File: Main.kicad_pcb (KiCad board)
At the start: 2 copper layers, 71.3 x 94.1 mm, 50 parts, among them J1 Conn_01x02, J10 Conn_01x04, J11 Conn_01x02, J12 Conn_01x02, J13 Conn_01x02, J14 Conn_01x02, J15 Conn_01x02, J2 Conn_01x02, J3 Conn_01x04, J4 Conn_01x02, J5 Conn_01x02, J6 Conn_01x08_Socket, J7 Conn_01x08_Socket, J8 Conn_01x08_Socket, J9 Conn_01x08_Socket, Q1 PMOS, Q2 SS8050, U1 DEV-16771, U2 K230D, U4 AP63201WU, U6 AP63201WU

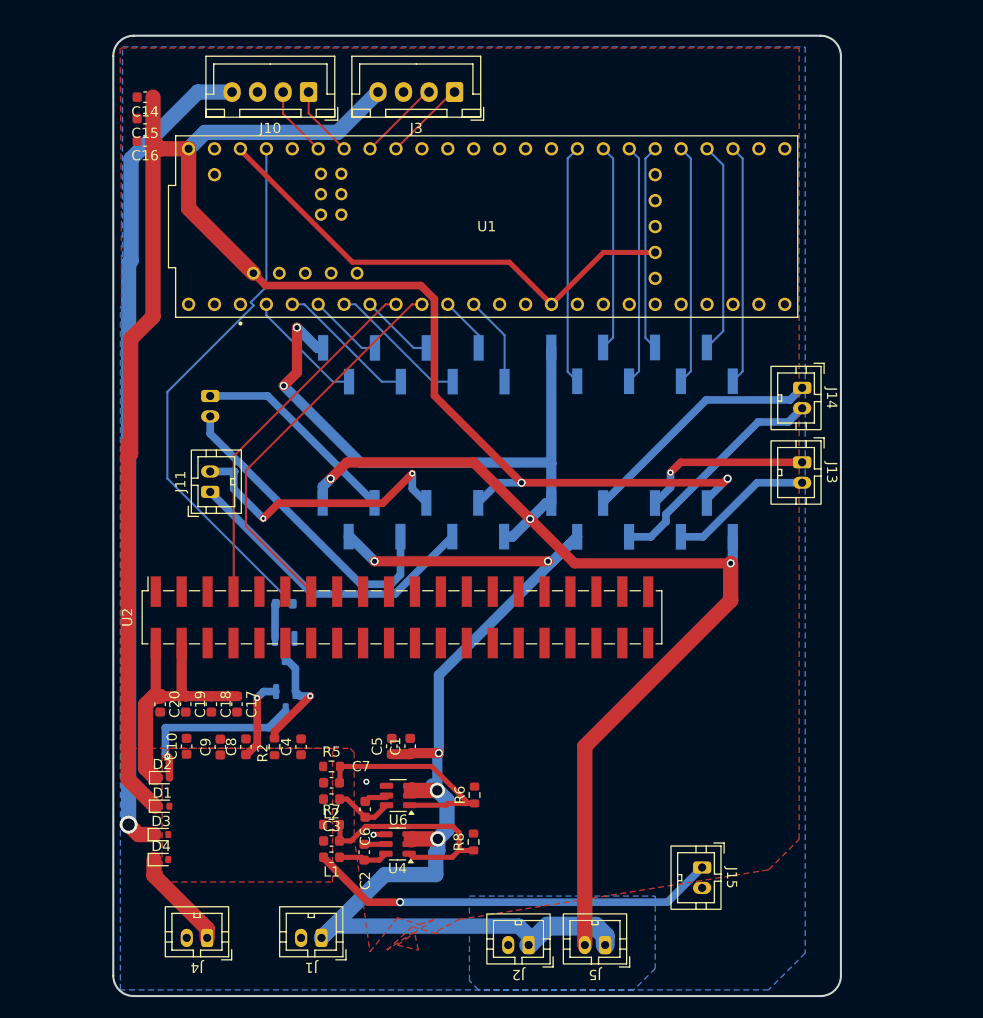
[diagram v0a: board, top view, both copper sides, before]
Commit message: Add files via upload
Please help make smaller!
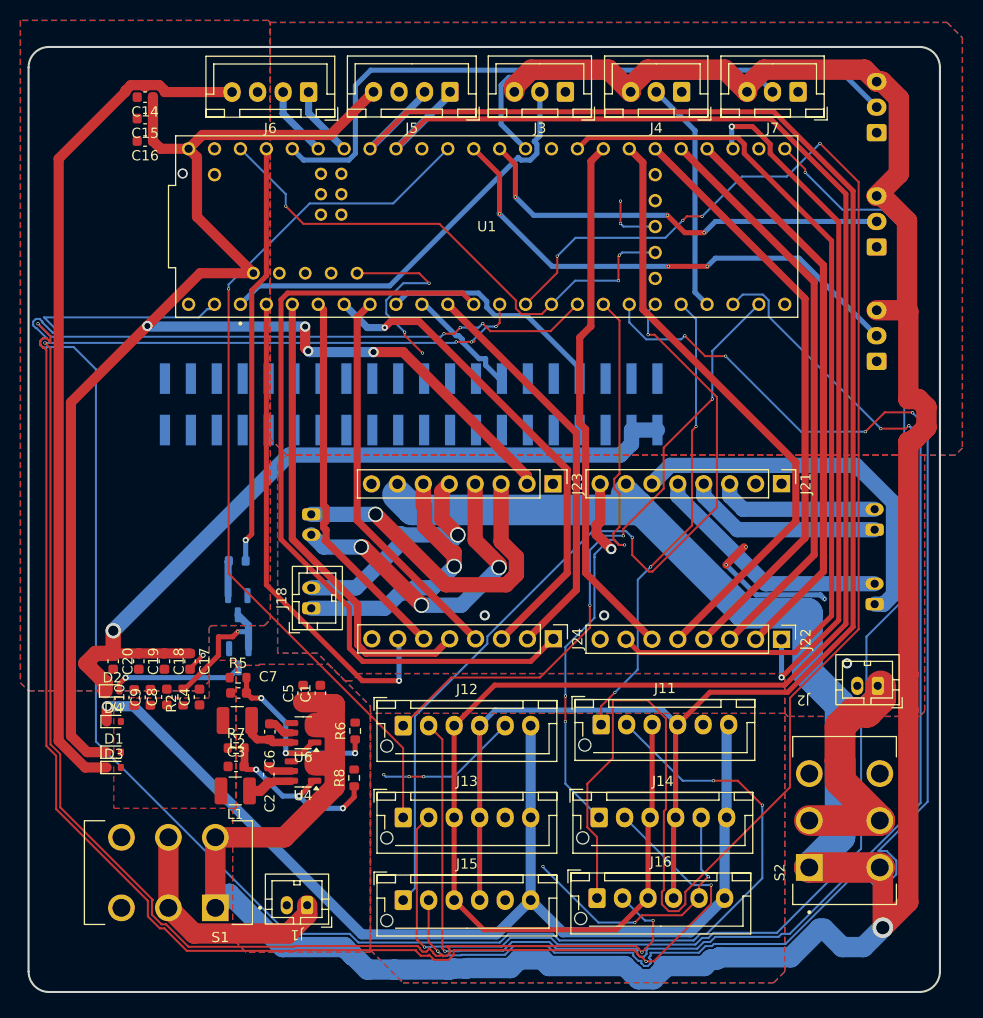
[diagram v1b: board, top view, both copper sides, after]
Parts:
- removed the J5 at (116.6, 132.4)
- added J10: Conn_01x03, Connector_JST:JST_XH_B3B-XH-A_1x03_P2.50mm_Vertical, B.Cu at (143.2, 52.8)
- added J11: Conn_01x06, Connector_JST:JST_XH_B6B-XH-AM_1x06_P2.50mm_Vertical, F.Cu at (116.2, 110.8)
- added J12: Conn_01x06, Connector_JST:JST_XH_B6B-XH-AM_1x06_P2.50mm_Vertical, F.Cu at (96.8, 110.9)
- added J13: Conn_01x06, Connector_JST:JST_XH_B6B-XH-AM_1x06_P2.50mm_Vertical, F.Cu at (96.8, 119.9)
- added J14: Conn_01x06, Connector_JST:JST_XH_B6B-XH-AM_1x06_P2.50mm_Vertical, F.Cu at (116.0, 119.9)
- added J16: Conn_01x06, Connector_JST:JST_XH_B6B-XH-AM_1x06_P2.50mm_Vertical, F.Cu at (115.8, 127.8)
- added J3: Conn_01x03, Connector_JST:JST_XH_B3B-XH-A_1x03_P2.50mm_Vertical, F.Cu at (112.7, 48.8)
- added J7: Conn_01x03, Connector_JST:JST_XH_B3B-XH-A_1x03_P2.50mm_Vertical, F.Cu at (135.5, 48.8)
- added J8: Conn_01x03, Connector_JST:JST_XH_B3B-XH-A_1x03_P2.50mm_Vertical, B.Cu at (143.2, 64.0)
- added J9: Conn_01x03, Connector_JST:JST_XH_B3B-XH-A_1x03_P2.50mm_Vertical, B.Cu at (143.2, 75.2)
- added S1: GF-126-0159, GF_126_0159:SW_GF-126-0159, F.Cu at (73.8, 125.3)
- added S2: GF-126-0159, GF_126_0159:SW_GF-126-0159, F.Cu at (140.1, 120.2)
- J15: value Conn_01x02 -> Conn_01x06; footprint Connector_TE-Connectivity:TE_440054-2_1x02_P2.00mm_Vertical -> Connector_JST:JST_XH_B6B-XH-AM_1x06_P2.50mm_Vertical
- J17: renamed from J11; moved to B.Cu
- J18: renamed from J12; moved to F.Cu
- J19: renamed from J13; moved to B.Cu
- J20: renamed from J14; moved to B.Cu
- J21: renamed from J8; footprint Connector_PinHeader_2.54mm:PinHeader_1x08_P2.54mm_Vertical_SMD_Pin1Left -> Connector_PinHeader_2.54mm:PinHeader_1x08_P2.54mm_Vertical; moved to F.Cu
- J22: renamed from J9; footprint Connector_PinHeader_2.54mm:PinHeader_1x08_P2.54mm_Vertical_SMD_Pin1Left -> Connector_PinHeader_2.54mm:PinHeader_1x08_P2.54mm_Vertical; moved to F.Cu
- J23: renamed from J6; footprint Connector_PinHeader_2.54mm:PinHeader_1x08_P2.54mm_Vertical_SMD_Pin1Left -> Connector_PinHeader_2.54mm:PinHeader_1x08_P2.54mm_Vertical; moved to F.Cu
- J24: renamed from J7; footprint Connector_PinHeader_2.54mm:PinHeader_1x08_P2.54mm_Vertical_SMD_Pin1Left -> Connector_PinHeader_2.54mm:PinHeader_1x08_P2.54mm_Vertical; moved to F.Cu
- J4: value Conn_01x02 -> Conn_01x03; footprint Connector_TE-Connectivity:TE_440054-2_1x02_P2.00mm_Vertical -> Connector_JST:JST_XH_B3B-XH-A_1x03_P2.50mm_Vertical
- L1, L2: footprint Inductor_SMD:L_0603_1608Metric -> Inductor_SMD:L_1210_3225Metric
- U2: moved to B.Cu
- moved J4 95.1 mm to (124.1, 48.8)
- moved J2 42.6 mm to (143.3, 107.0)
- moved J22 30.2 mm to (133.9, 102.4), turned to -90 degrees
- moved J24 30.1 mm to (111.5, 102.4), turned to -90 degrees
- moved J15 29.5 mm to (96.8, 128.0), turned to 0 degrees
- moved J18 23.0 mm to (87.8, 99.4), turned to 90 degrees
- moved J20 22.4 mm to (143.0, 99.0), turned to 90 degrees
- moved U2 20.9 mm to (97.6, 79.4)
- moved D4 14.3 mm to (68.5, 110.5)
- moved J21 14.1 mm to (133.9, 87.2), turned to -90 degrees
- moved J23 14.1 mm to (111.5, 87.2), turned to -90 degrees
- moved R6 13.3 mm to (92.1, 111.4)
- moved R8 13.3 mm to (92.0, 116.0)
- moved C7 12.7 mm to (80.7, 107.7)
- moved R5 12.6 mm to (80.6, 106.2)
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- renumbered J3 to J5, J10 to J6
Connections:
- J1 pad 1: +6.6V -> Net-(J1-Pin_1)
- J15 pad 1: +5.3V -> /X5
- J15 pad 2: GND -> /G5
- J2 pad 1: +6.6V -> Net-(J2-Pin_1)
- J4 pad 1: Net-(D4-K) -> GND
- J4 pad 2: GND -> /KRS2
- U1 pad 0: unconnected-(U1-RX1-Pad0) -> /G1
- U1 pad 1: unconnected-(U1-TX1-Pad1) -> /KRS1
- U1 pad 11: unconnected-(U1-MOSI-Pad11) -> /G6
- U1 pad 12: unconnected-(U1-MISO-Pad12) -> /X6
- U1 pad 13: unconnected-(U1-SCK-Pad13) -> /L1
- U1 pad 14: unconnected-(U1-A0-Pad14) -> /L2
- U1 pad 15: unconnected-(U1-A1-Pad15) -> /L3
- U1 pad 16: unconnected-(U1-A2-Pad16) -> /X3
- U1 pad 22: unconnected-(U1-A8-Pad22) -> /L4
- U1 pad 24: unconnected-(U1-A10-Pad24) -> /G4
- U1 pad 25: unconnected-(U1-A11-Pad25) -> /X4
- U1 pad 26: unconnected-(U1-A12-Pad26) -> /G5
- U1 pad 27: unconnected-(U1-A13-Pad27) -> /X5
- U1 pad 28: unconnected-(U1-RX7-Pad28) -> /X1
- U1 pad 29: unconnected-(U1-TX7-Pad29) -> /KRS2
- U1 pad 30: unconnected-(U1-CRX3-Pad30) -> /G2
- U1 pad 31: unconnected-(U1-CTX3-Pad31) -> /X2
- U1 pad 33: unconnected-(U1-MCLK2-Pad33) -> /G3
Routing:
- net +6.6V: track 119.9 -> 338.8 mm, vias 5 -> 1
- net /G4: track 0.00 -> 193.5 mm, vias 0 -> 6
- net /SDA: track 8.04 -> 196.5 mm
- net /SCL: track 8.08 -> 178.6 mm
- net /G1: track 0.00 -> 169.3 mm, vias 0 -> 2
- net /X6: track 0.00 -> 167.5 mm, vias 0 -> 4
- net /G6: track 0.00 -> 167.2 mm, vias 0 -> 6
- net /G5: track 0.00 -> 142.6 mm, vias 0 -> 5
- net /G2: track 0.00 -> 140.5 mm, vias 0 -> 3
- net /G3: track 0.00 -> 138.3 mm, vias 0 -> 2
- net MGND: track 153.0 -> 20.9 mm, vias 5 -> 7
- net Net-(D4-K): track 9.83 -> 109.6 mm, vias 0 -> 1
- net /X3: track 0.00 -> 86.3 mm, vias 0 -> 1
- net /X5: track 0.00 -> 84.7 mm, vias 0 -> 2
- net /PWMA: track 8.83 -> 78.0 mm
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- added copper zone on F.Cu, net MGND
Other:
- board size 71.3 x 94.1 mm -> 89.3 x 92.6 mm
